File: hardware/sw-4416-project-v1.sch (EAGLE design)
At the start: 30 parts, among them IC1 MCP73831, U1 V_REG_317SMD, X1 USB-MICROB

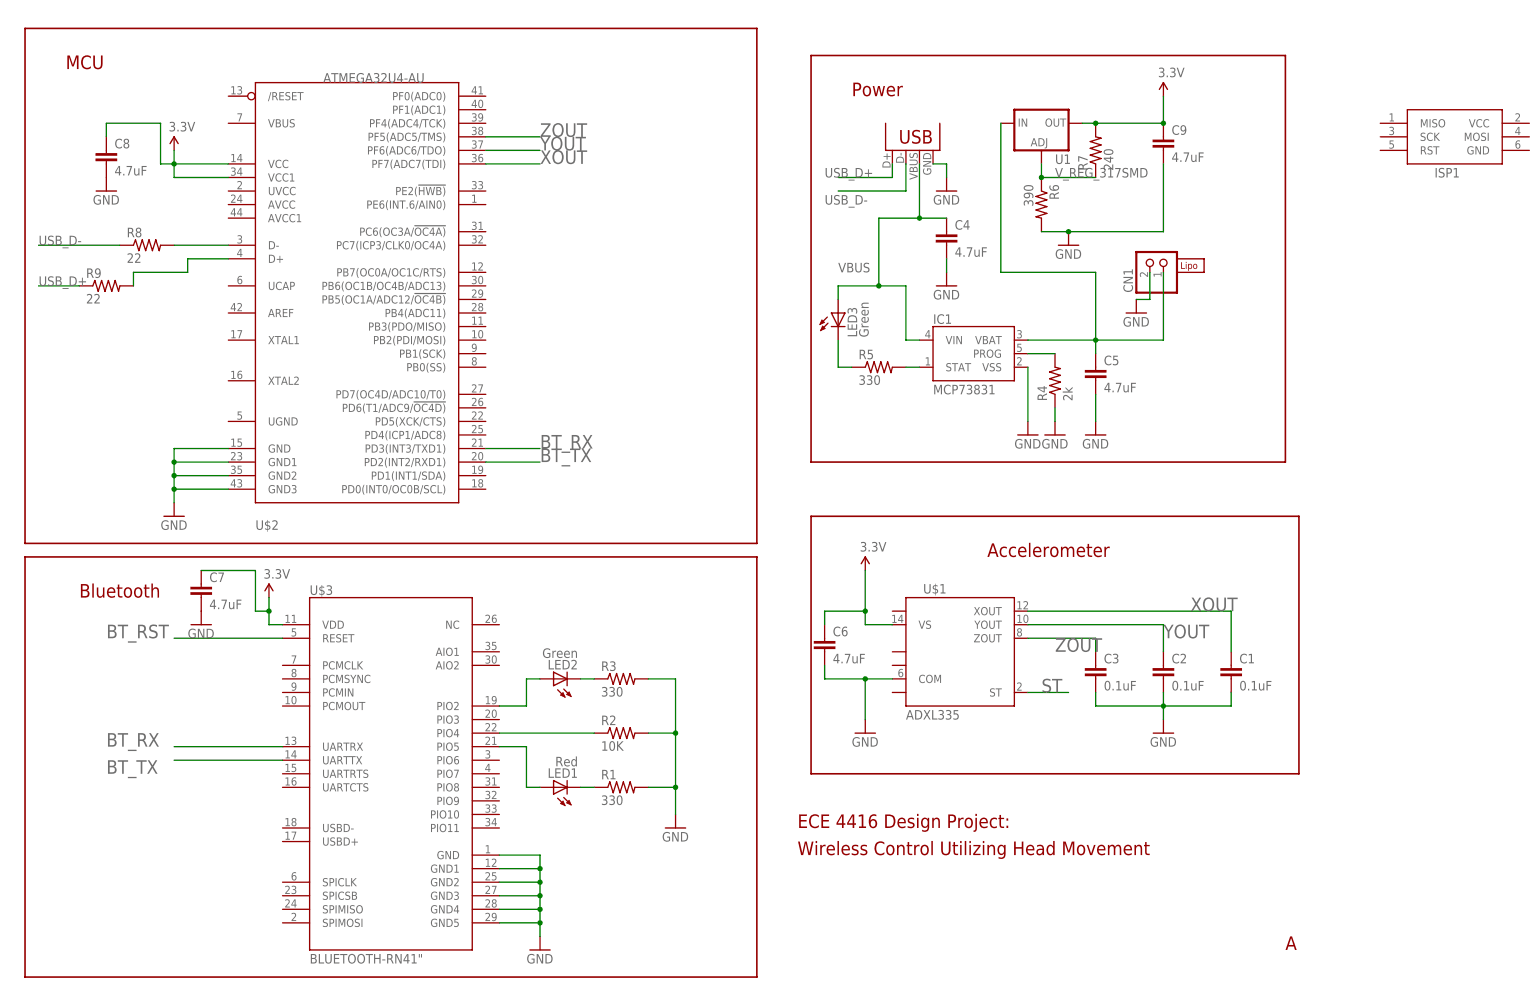
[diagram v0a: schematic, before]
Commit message: schematic version 1 completed
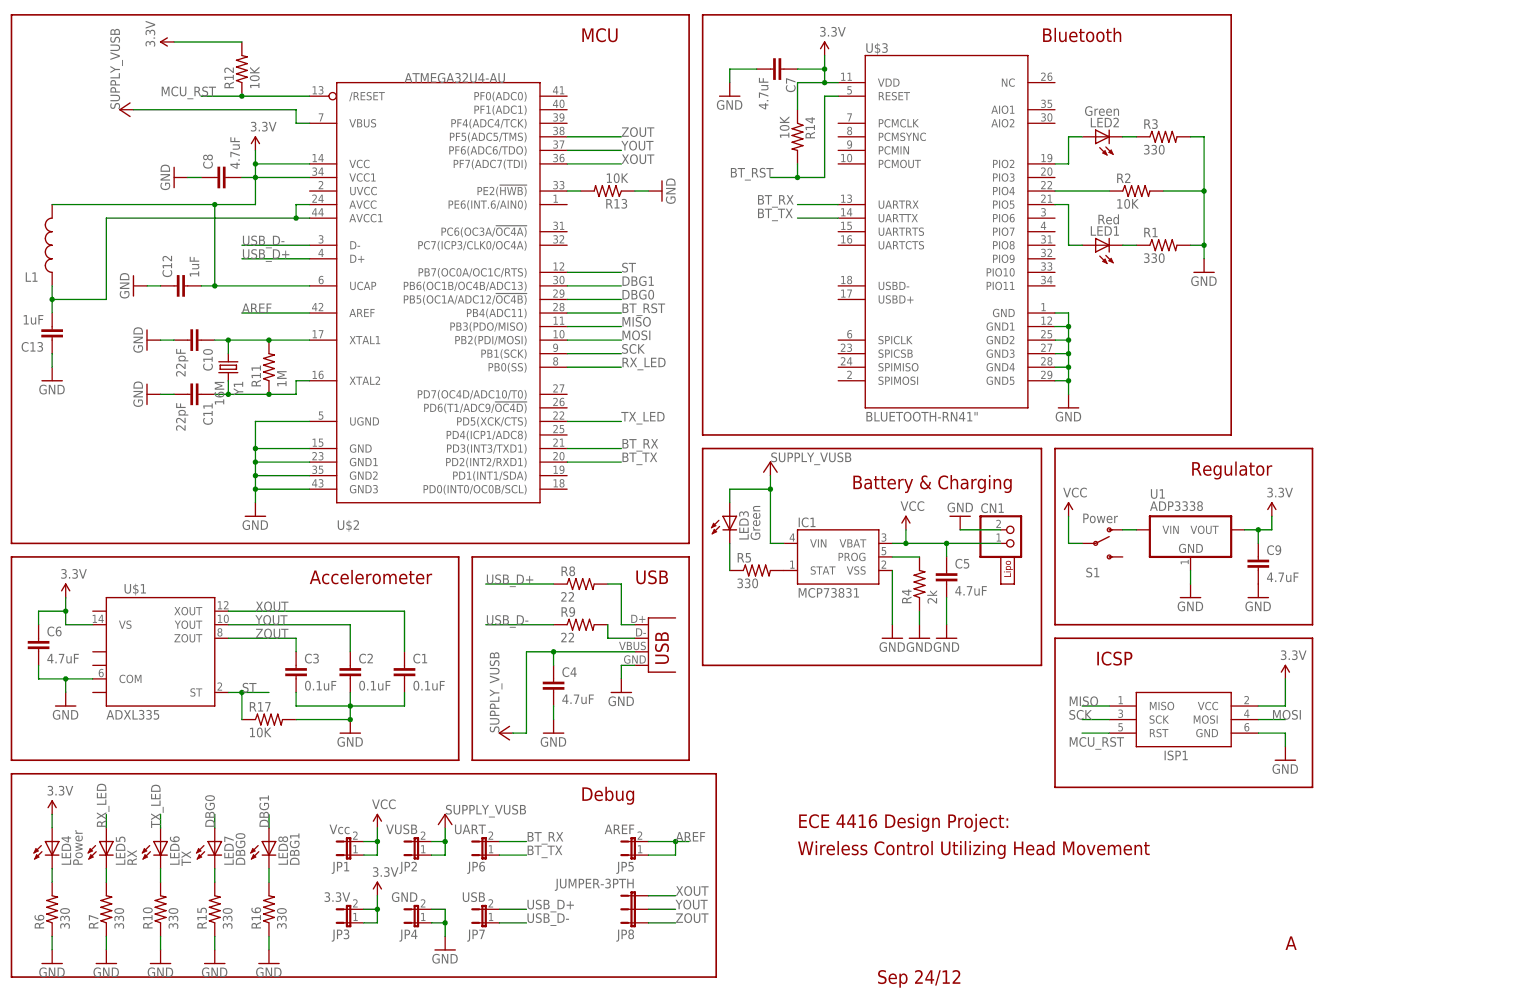
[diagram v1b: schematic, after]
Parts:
- added C10, C11: 22pF, SparkFun:CAP0603-CAP
- added C12, C13: 1uF, SparkFun:CAP0603-CAP
- added JP1: Vcc, SparkFun:JUMPER-2PTH
- added JP2: VUSB, SparkFun:JUMPER-2PTH
- added JP3: 3.3V, SparkFun:JUMPER-2PTH
- added JP4: GND, SparkFun:JUMPER-2PTH
- added JP5: AREF, SparkFun:JUMPER-2PTH
- added JP6: UART, SparkFun:JUMPER-2PTH
- added JP7: USB, SparkFun:JUMPER-2PTH
- added JP8: JUMPER-3PTH, SparkFun:JUMPER-3PTH
- added L1: (no value), SparkFun:INDUCTOR0805
- added LED4: Power, SparkFun:LED0603
- added LED5: RX, SparkFun:LED0603
- added LED6: TX, SparkFun:LED0603
- added LED7: DBG0, SparkFun:LED0603
- added LED8: DBG1, SparkFun:LED0603
- added R10, R15, R16: 330, SparkFun:RESISTOR0603-RES
- added R11: 1M, SparkFun:RESISTOR0603-RES
- added R12, R13, R14, R17: 10K, SparkFun:RESISTOR0603-RES
- added S1: Power, SparkFun:SWITCH-SPST-SMD-A
- added Y1: 16M, SparkFun:CRYSTALHC49US
- R6: value 390 -> 330
- R7: value 240 -> 330
- U1: value V_REG_317SMD -> ADP3338; device SparkFun:V_REG_317SMD -> dp_devices:VREG_3PINS-SOT-223
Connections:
- removed net VBUS: C4.1, IC1.VIN, LED3.A, X1.VBUS
- new net AREF: JP5.1, JP5.2, U$2.AREF
- new net DBG0: LED7.A, U$2.PB5(OC1A/ADC12/!OC4B)
- new net DBG1: LED8.A, U$2.PB6(OC1B/OC4B/ADC13)
- new net MCU_RST: ISP1.RST, R12.1, U$2./RESET
- new net MISO: ISP1.MISO, U$2.PB3(PDO/MISO)
- new net MOSI: ISP1.MOSI, U$2.PB2(PDI/MOSI)
- new net N$13: C10.1, R11.2, U$2.XTAL1, Y1.1
- new net N$14: C11.1, R11.1, U$2.XTAL2, Y1.2
- new net N$15: R8.2, X1.D+
- new net N$16: LED7.C, R15.2
- new net N$17: C13.2, L1.1, U$2.AVCC, U$2.AVCC1
- new net N$18: LED8.C, R16.2
- new net N$19: R13.2, U$2.PE2(!HWB)
- new net N$20: R9.2, X1.D-
- new net RX_LED: LED5.A, U$2.PB0(SS)
- new net SCK: ISP1.SCK, U$2.PB1(SCK)
- new net TX_LED: LED6.A, U$2.PD5(XCK/CTS)
- new net VUSB: C4.1, IC1.VIN, JP2.1, JP2.2, LED3.A, U$2.VBUS, X1.VBUS
- net 3.3V: now also C12.2, C6.1, C7.1, C8.2, ISP1.VCC, JP3.1, JP3.2, L1.2, LED4.A, R12.2, R14.1, U$1.VS@14, U$2.UCAP, U$2.VCC, U$2.VCC1, U$3.VDD, U1.VOUT; no longer R7.2, U1.OUT
- net BT_RST: now also R14.2, U$2.PB4(ADC11)
- net BT_RX: now also JP6.2
- net BT_TX: now also JP6.1
- net GND: now also C10.2, C11.2, C12.1, C13.1, C8.1, ISP1.GND, JP4.1, JP4.2, R10.1, R13.1, R15.1, R16.1, R17.2, R6.1, R7.1, U$2.UGND, U1.GND; no longer C8.2, R6.2
- net N$10: now also LED5.C, R7.2; no longer R8.2, U$2.D-
- net N$11: now also S1.O, U1.VIN; no longer C5.1, CN1.2, IC1.VBAT, U1.IN
- net N$12: now also LED6.C, R10.2; no longer R6.1, R7.1, U1.ADJ
- net N$9: now also LED4.C, R6.2; no longer R9.2, U$2.D+
- net ST: now also R17.1, U$2.PB7(OC0A/OC1C/RTS)
- net USB_D+: now also JP7.2, R8.1, U$2.D+; no longer R9.1, X1.D+
- net USB_D-: now also JP7.1, R9.1, U$2.D-; no longer R8.1, X1.D-
- net VCC: now also C5.1, CN1.2, IC1.VBAT, JP1.1, JP1.2, S1.P; no longer C6.1, C7.1, C8.1, U$1.VS@14, U$2.VCC, U$2.VCC1, U$3.VDD
- net XOUT: now also JP8.3
- net YOUT: now also JP8.2
- net ZOUT: now also JP8.1
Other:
- note added: "Battery & Charging"
- note added: "Debug"
- note added: "ICSP"
- note added: "Regulator"
- note added: "Sep 24/12"
- note added: "USB"
- note removed: "Power"
- moved on the sheet: C1, C2, C3, C4, C5, C6, C7, C8, C9, CN1, IC1, ISP1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
